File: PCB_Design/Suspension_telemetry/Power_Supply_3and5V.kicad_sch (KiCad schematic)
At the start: 21 parts, among them IC1 MCP73844-840I_MS, Q1 SI4435DY, U2 LMR62421XMF

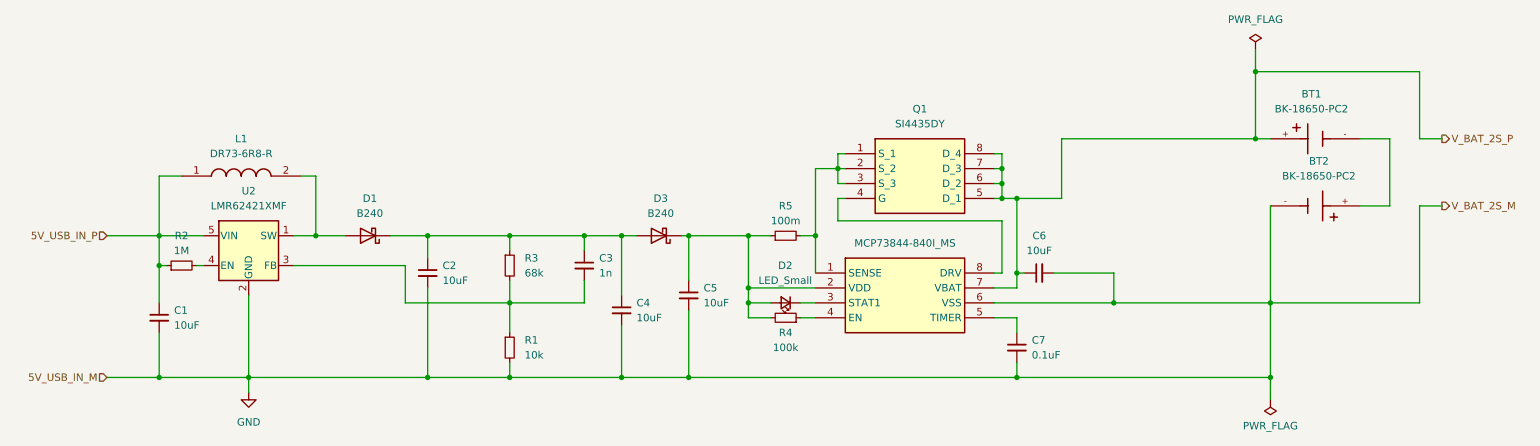
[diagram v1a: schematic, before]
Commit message: pcv v2 finished
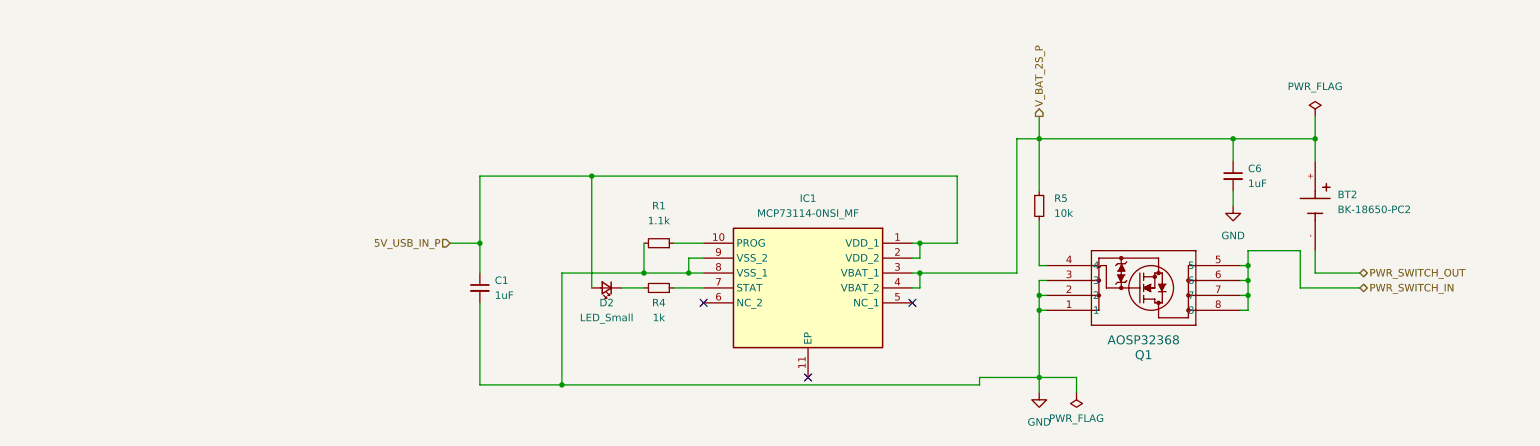
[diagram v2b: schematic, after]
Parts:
- removed BT1: BK-18650-PC2, BAT_BK-18650-PC2:BAT_BK-18650-PC2, symbol BK-18650-PC2:BK-18650-PC2
- removed C2, C4, C5: 10uF, Capacitor_SMD:C_0603_1608Metric_Pad1.08x0.95mm_HandSolder, symbol Device:C_Small
- removed C3: 1n, Capacitor_SMD:C_0603_1608Metric_Pad1.08x0.95mm_HandSolder, symbol Device:C_Small
- removed C7: 0.1uF, Capacitor_SMD:C_0603_1608Metric_Pad1.08x0.95mm_HandSolder, symbol Device:C_Small
- removed D1, D3: B240, Diode_SMD:D_SMB, symbol Diode:B240
- removed IC1: MCP73844-840I_MS, SOP65P490X110-8N:SOP65P490X110-8N, symbol MCP73844-840I_MS:MCP73844-840I_MS
- removed L1: DR73-6R8-R, INDM7676X355N:INDM7676X355N, symbol DR73-6R8-R:DR73-6R8-R
- removed Q1: SI4435DY, SOIC127P600X175-8N:SOIC127P600X175-8N, symbol SI4435DY:SI4435DY
- removed R2: 1M, Resistor_SMD:R_0603_1608Metric_Pad0.98x0.95mm_HandSolder, symbol Device:R_Small
- removed R3: 68k, Resistor_SMD:R_0603_1608Metric_Pad0.98x0.95mm_HandSolder, symbol Device:R_Small
- removed U2: LMR62421XMF, Package_TO_SOT_SMD:SOT-23-5, symbol Regulator_Switching:LMR62421XMF
- added IC1: MCP73114-0NSI_MF, SON50P300X300X100-11N-D, symbol MCP73114:MCP73114-0NSI_MF
- added Q1: AOSP32368, SO8SOP-8L_AOS, symbol AOSP_TELEMETRY_REVERSE_POLARITY:AOSP32368
- C1, C6: value 10uF -> 1uF
- R1: value 10k -> 1.1k
- R4: value 100k -> 1k
- R5: value 100m -> 10k
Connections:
- net 5V_USB_IN_P: now also D2.2 (A), IC1.1 (VDD_1), IC1.2 (VDD_2)
- net GND: now also IC1.8 (VSS_1), IC1.9 (VSS_2), Q1.1, Q1.2, Q1.3; no longer BT2.-
- net V_BAT_2S_P: now also BT2.+, R5.1, IC1.3 (VBAT_1), IC1.4 (VBAT_2)
- net at R1.1: now also IC1.10 (PROG)
- net at D2.1 (K): now also R4.2
- net at R5.2: now also Q1.4
- net at R4.1: now also IC1.7 (STAT)
- new net PWR_SWITCH_IN: Q1.5, Q1.6, Q1.7, Q1.8
- new net PWR_SWITCH_OUT: BT2.-
- no-connect marks 0 -> 3
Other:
- moved on the sheet: BT2, D2, R4, R5
